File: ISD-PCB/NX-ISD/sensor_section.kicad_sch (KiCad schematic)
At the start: 22 parts, among them U10 BNO085, U12 OPT3001DNPR, U3 MAX17048G_T10, U4 RV-3028-C7, U5 MAX30102, U6 BME690, Y2 32.768

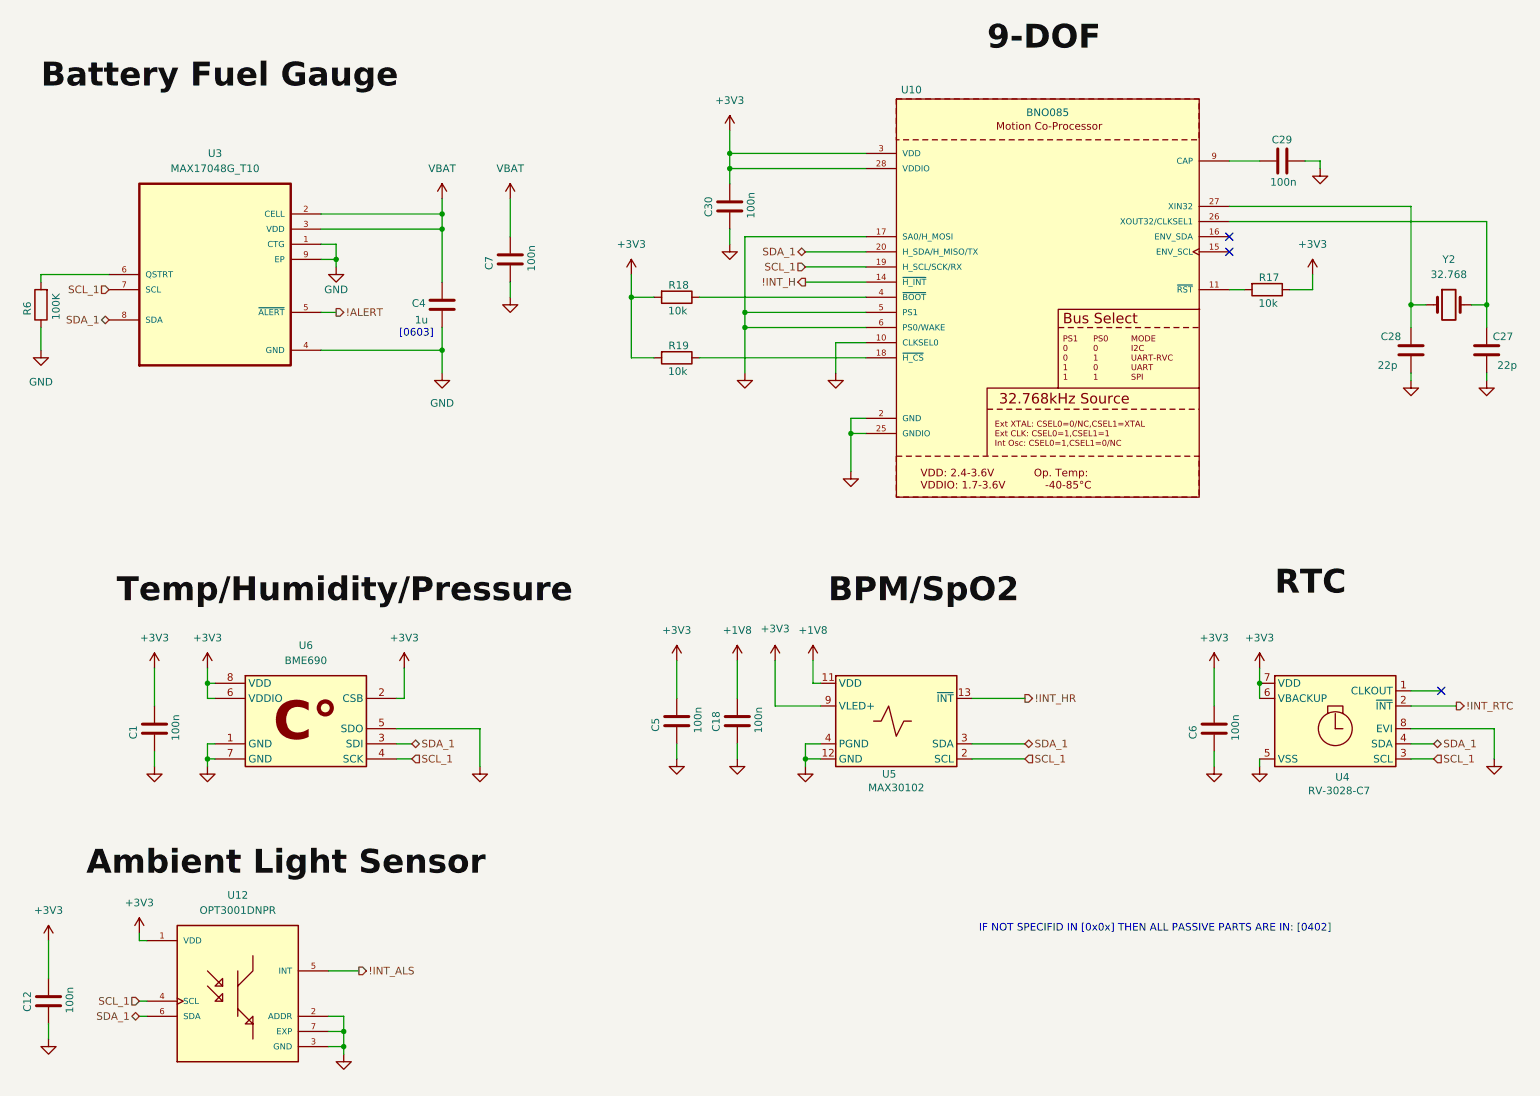
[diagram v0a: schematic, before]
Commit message: v1p3 major fix rework in progress
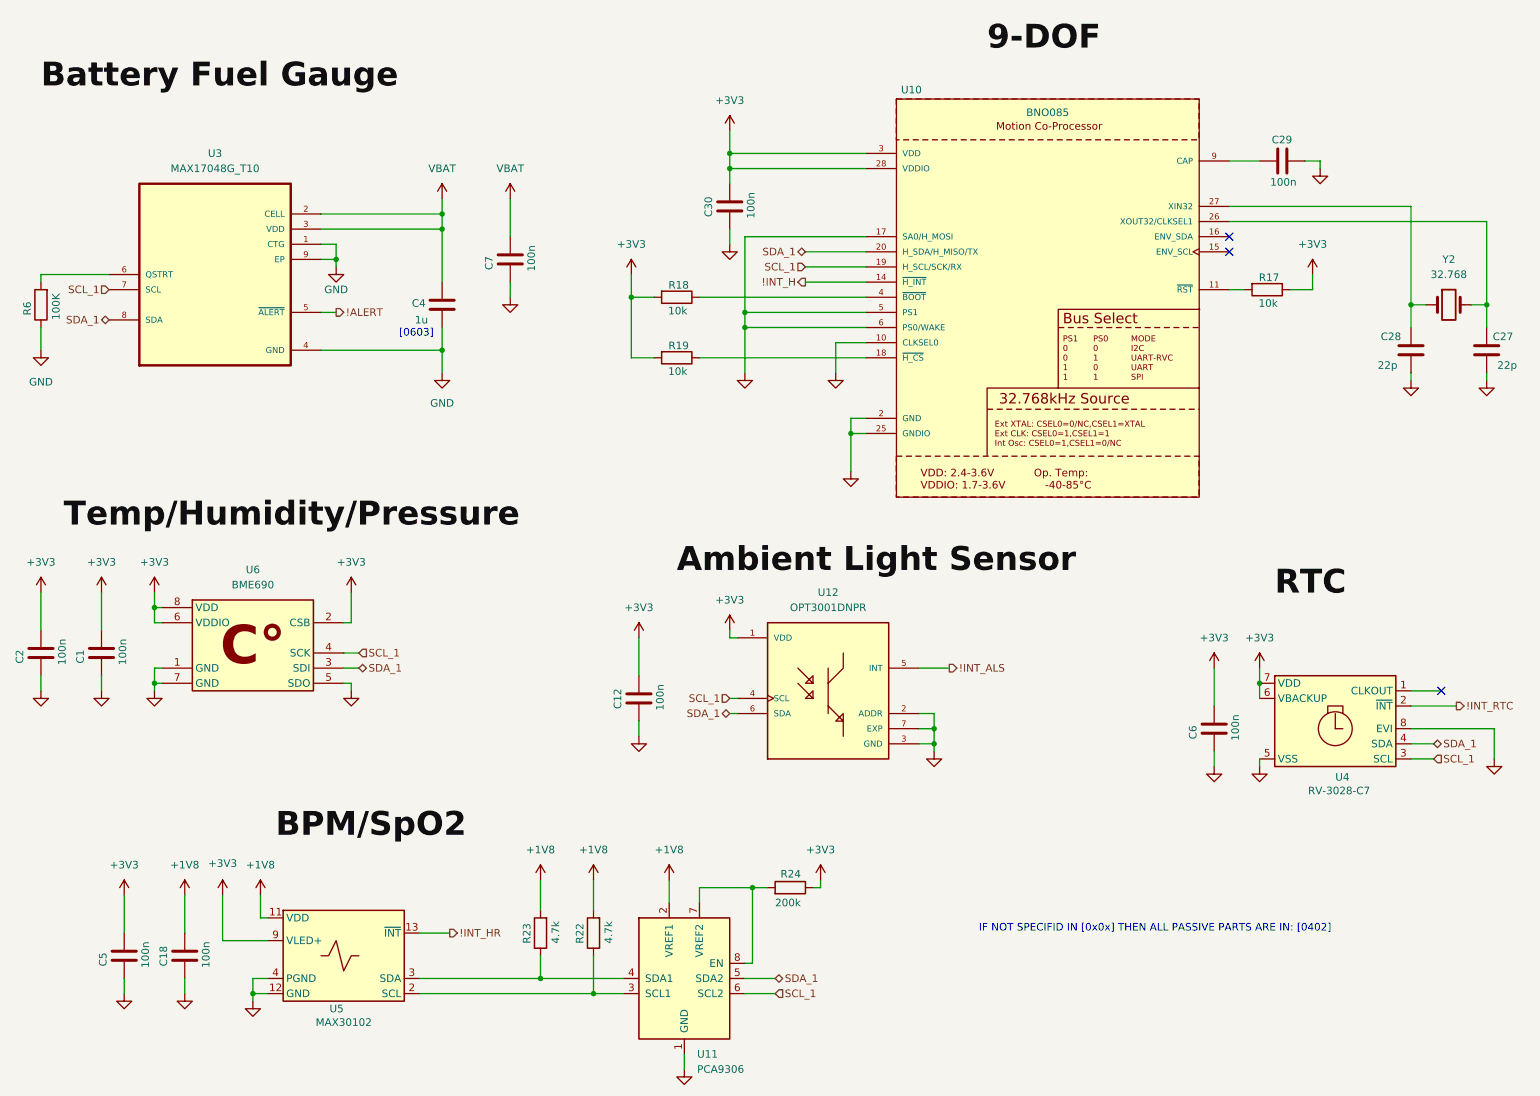
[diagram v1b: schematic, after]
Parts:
- added C2: 100n, Capacitor_SMD:C_0402_1005Metric, symbol Device:C
- added R22, R23: 4.7k, Resistor_SMD:R_0402_1005Metric, symbol Device:R
- added R24: 200k, Resistor_SMD:R_0402_1005Metric, symbol Device:R
- added U11: PCA9306, Package_SO:VSSOP-8_2.3x2mm_P0.5mm, symbol Interface:PCA9306
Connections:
- net +1V8: now also R22.2, R23.2, U11.2 (VREF1)
- net +3V3: now also C2.1, R24.1
- net GND: now also C2.2, U11.1 (GND)
- net SCL_1: now also U11.6 (SCL2); no longer U5.2 (SCL)
- net SDA_1: now also U11.5 (SDA2); no longer U5.3 (SDA)
- new net: R22.1, U11.3 (SCL1), U5.2 (SCL)
- new net: R23.1, U11.4 (SDA1), U5.3 (SDA)
- new net: R24.2, U11.7 (VREF2), U11.8 (EN)
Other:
- moved on the sheet: C1, C12, C18, C5, U12, U5, U6

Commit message: Added 3D-Renders to README
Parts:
- U12: footprint NX-AW-footprints:SON65P200X200X65-7N -> Global Footprints:SON65P200X200X65-7N
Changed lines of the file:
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@@
 			)
 		)
-		(property "Footprint" "NX-AW-footprints:SON65P200X200X65-7N"
+		(property "Footprint" "Global Footprints:SON65P200X200X65-7N"
 			(at 156.21 129.54 0)
 			(hide yes)
